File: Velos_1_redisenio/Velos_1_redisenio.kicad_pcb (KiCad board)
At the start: 2 copper layers, 104.3 x 59.6 mm, 28 parts, among them J1 conector_motor, J2 S_Bus, J3 llave_habilitacion, J4 parada_emergencia, J5 V_in +9VDC, J6 Control Driver, J7 potenciometro, K1 Relay_SPDT, Q1 BC548, Q2 BC548, Q3 BC548, Q4 BC548, Q5 BC548, U1 LM358, U2 L7805

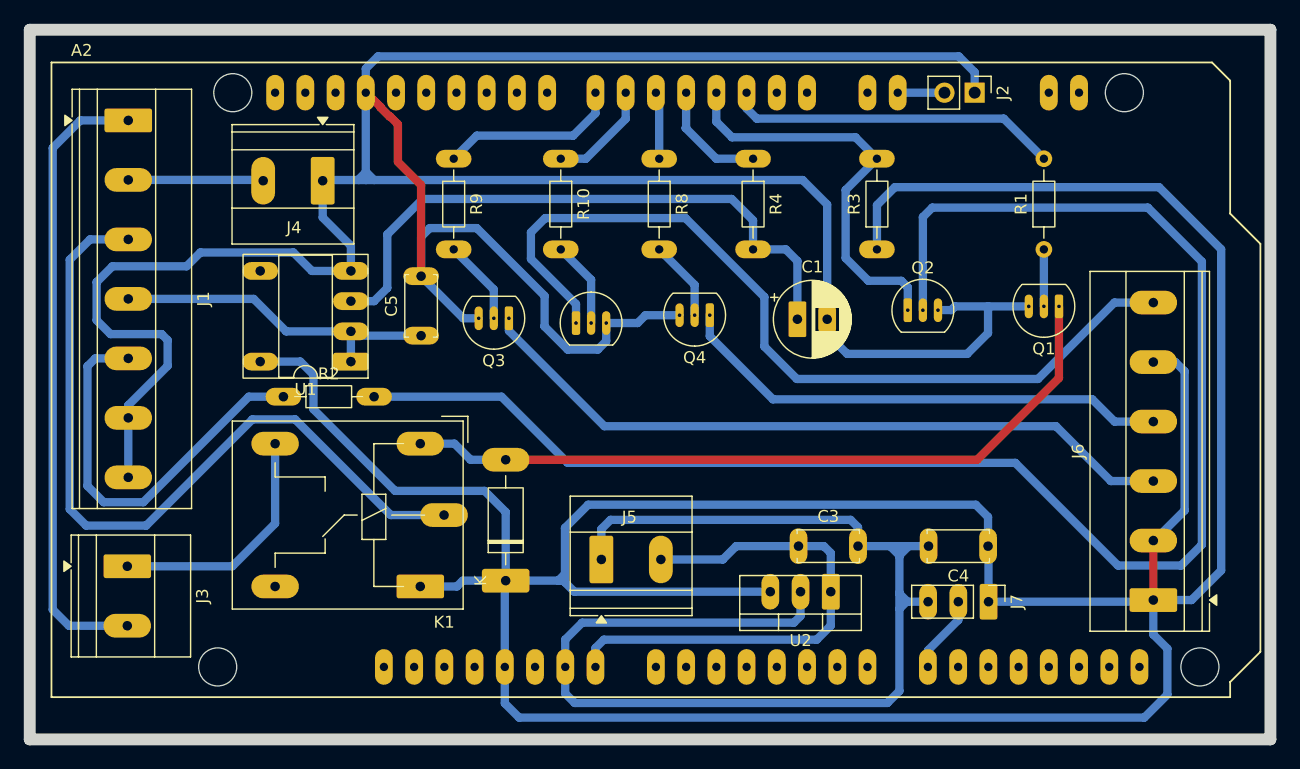
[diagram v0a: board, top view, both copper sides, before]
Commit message: placa
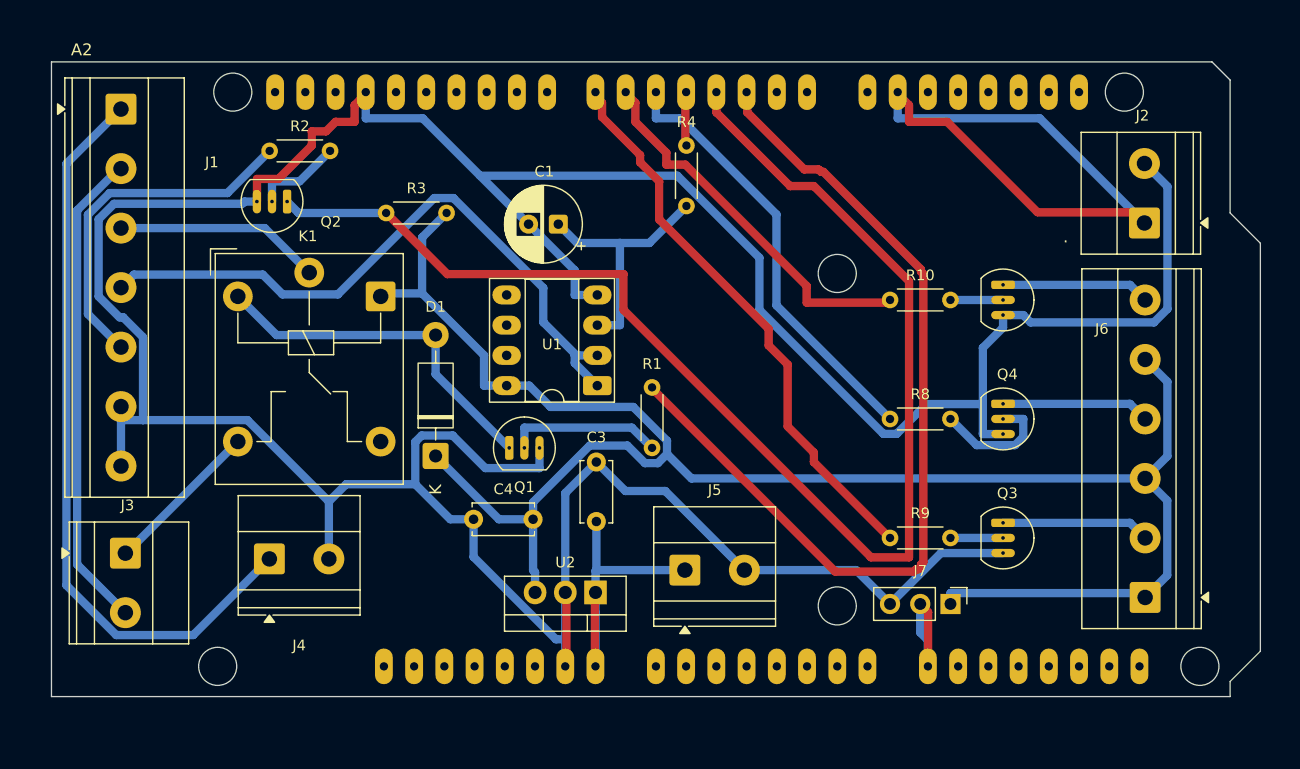
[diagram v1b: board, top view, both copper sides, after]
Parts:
- removed C5: 100nF, Capacitor_THT:C_Disc_D5.0mm_W2.5mm_P5.00mm
- A2: footprint footprints:Arduino_Mega2560_Shield -> Velos_Local:Arduino_Mega2560_Shield
- D1: footprint Diode_THT:D_DO-41_SOD81_P10.16mm_Horizontal -> Velos_Local:D_DO41_Local
- J2: footprint Connector_PinHeader_2.54mm:PinHeader_1x02_P2.54mm_Vertical -> TerminalBlock_Phoenix:TerminalBlock_Phoenix_MKDS-1,5-2_1x02_P5.00mm_Horizontal
- Q1: footprint Package_TO_SOT_THT:TO-92_Inline -> Velos_Local:BC548_THT_Q1
- Q2: footprint Package_TO_SOT_THT:TO-92_Inline -> Velos_Local:BC548_THT_Q2
- Q3: footprint Package_TO_SOT_THT:TO-92_Inline -> Velos_Local:BC548_THT_Q3
- Q4: footprint Package_TO_SOT_THT:TO-92_Inline -> Velos_Local:BC548_THT_Q4
- Q5: footprint Package_TO_SOT_THT:TO-92_Inline -> Velos_Local:BC548_THT_Q5
- R1, R10, R2, R3, R4, R8, R9: footprint Resistor_THT:R_Axial_DIN0204_L3.6mm_D1.6mm_P7.62mm_Horizontal -> Resistor_THT:R_Axial_DIN0204_L3.6mm_D1.6mm_P5.08mm_Horizontal
- moved Q2 53.0 mm to (128.3, 70.3), turned to 180 degrees
- moved R9 48.6 mm to (179.0, 98.6), turned to 0 degrees
- moved Q1 47.7 mm to (147.0, 91.0), turned to 0 degrees
- moved Q3 44.9 mm to (188.5, 97.3), turned to -90 degrees
- moved C4 38.3 mm to (149.0, 97.0)
- moved R1 36.9 mm to (159.0, 91.0)
- moved R3 36.3 mm to (141.7, 71.3), turned to 180 degrees
- moved Q5 36.0 mm to (188.5, 77.3), turned to -90 degrees
- moved J4 32.1 mm to (126.8, 100.3), turned to 0 degrees
- moved R10 30.1 mm to (179.0, 78.6), turned to 0 degrees
- moved R8 29.2 mm to (179.0, 88.6), turned to 0 degrees
- moved Q4 25.8 mm to (188.5, 87.3), turned to -90 degrees
- moved K1 24.6 mm to (136.2, 78.3), turned to -90 degrees
- moved C1 21.6 mm to (151.1, 72.2), turned to 180 degrees
- moved U1 20.8 mm to (154.4, 85.8)
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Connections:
- A2 pad 5V1: +5V -> unconnected-(A2-5V-Pad5V1)
- A2 pad A0: unconnected-(A2-PadA0) -> Ref vel_D
- J1 pad 1: /Power_on_motor -> /Seguridad
- J1 pad 2: /Seguridad -> /Power_on_motor
- J2 pad 1: GND -> S-BUS
- J2 pad 2: S-BUS -> GND
- J4 pad 1: GND -> /Seguridad
- J4 pad 2: /Seguridad -> GND
- J5 pad 1: GND -> +9V
- J5 pad 2: +9V -> GND
- J6 pad 2: +5V -> Net-(J6-Pin_2)
- J6 pad 3: Net-(J6-Pin_3) -> +5V
- Q3 pad 1: Net-(J6-Pin_3) -> Net-(J6-Pin_2)
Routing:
- net +5V: track 294.7 -> 153.3 mm
- net Net-(Q2-B): track 133.5 -> 7.64 mm
- net Net-(A2-D3_INT1): track 34.8 -> 113.5 mm
- net Net-(J6-Pin_3): track 60.4 -> 0.00 mm
- net Net-(J6-Pin_6): track 72.7 -> 12.5 mm
- net /Seguridad: track 11.4 -> 63.4 mm
- net GND: track 364.3 -> 312.5 mm
- net S-BUS: track 3.93 -> 52.9 mm
- net Net-(J1-Pin_3): track 65.7 -> 17.4 mm
- net Net-(A2-D2_INT0): track 28.1 -> 76.2 mm
- net Net-(D1-A): track 63.1 -> 30.0 mm
- net Puls: track 15.2 -> 47.8 mm
- net Dir: track 5.66 -> 36.8 mm
- net Net-(U1A-+): track 52.2 -> 21.5 mm
- net Net-(J6-Pin_4): track 42.0 -> 12.5 mm
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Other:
- board size 104.3 x 59.6 mm -> 101.6 x 53.3 mm
